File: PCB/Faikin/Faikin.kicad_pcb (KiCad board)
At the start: 2 copper layers, 70 x 70 mm, 27 parts, among them J1 1x5, J3 USB-PROG, Q1 BSS138PS, U3 MD8942, U4 ESP32-S3-MINI-1

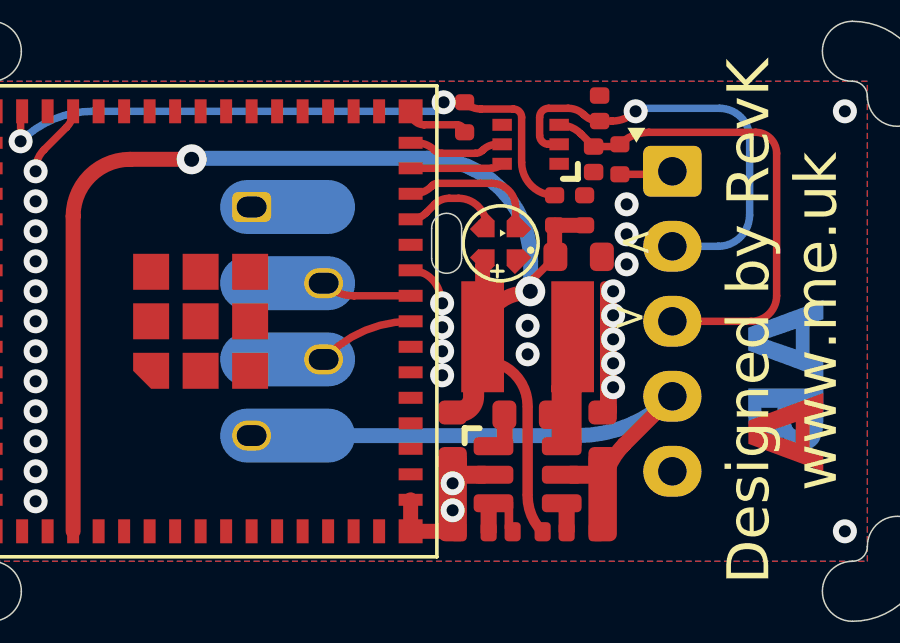
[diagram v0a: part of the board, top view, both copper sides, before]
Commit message: TC2030
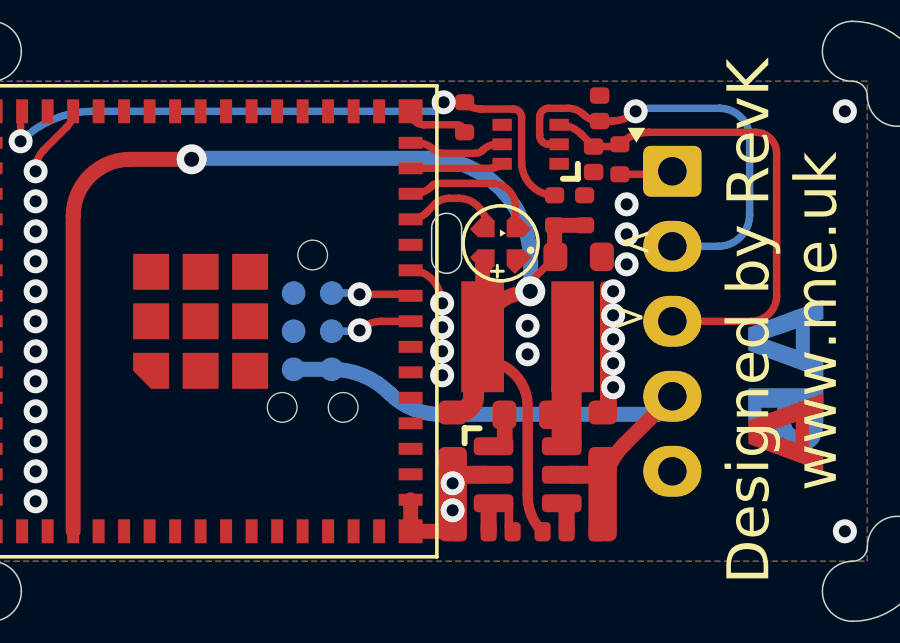
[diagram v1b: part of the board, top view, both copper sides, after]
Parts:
- removed J3: USB-PROG, RevK:USB-PROG2
- added J2: Conn_01x06, RevK:Tag-Connect_TC2030-IDC-NL_2x03_P1.27mm_Vertical, B.Cu at (138.7, 65.3)
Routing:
- net DC: track 16.1 -> 17.5 mm
- net D-: track 3.07 -> 2.72 mm, vias 0 -> 1
- net D+: track 3.01 -> 2.68 mm, vias 0 -> 1
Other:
- board text added: "B"

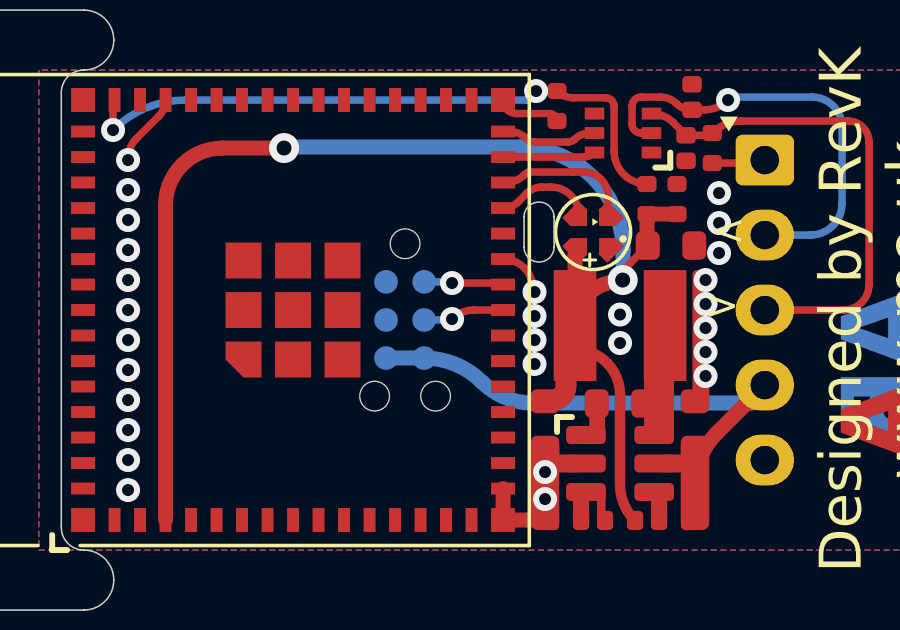
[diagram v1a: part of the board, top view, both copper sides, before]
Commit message: TC2030-USB-NL cable pin out
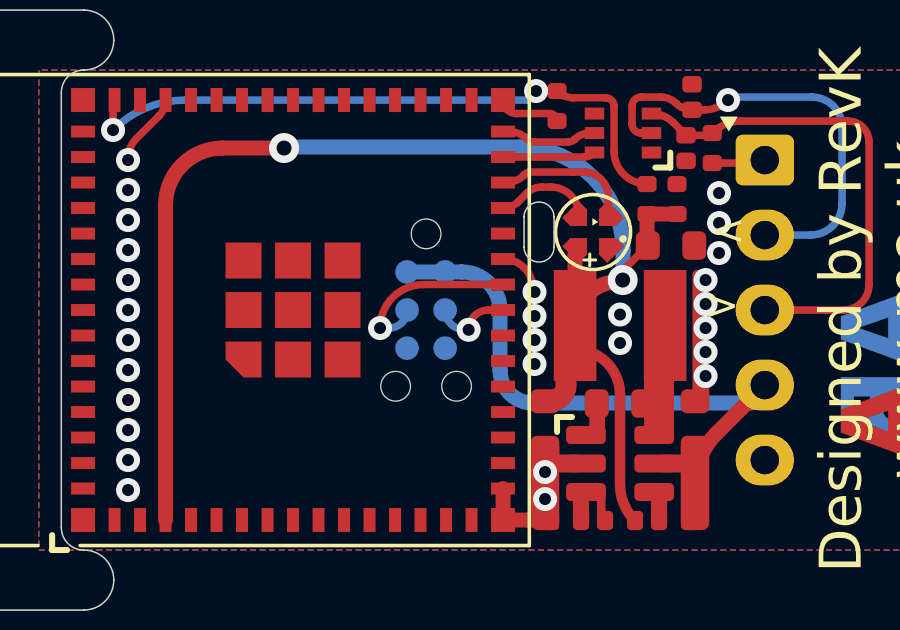
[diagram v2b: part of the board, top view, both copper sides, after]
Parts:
- removed J2: Conn_01x06, RevK:Tag-Connect_TC2030-IDC-NL_2x03_P1.27mm_Vertical
- added J3: TC2030-USB-NL, RevK:Tag-Connect_TC2030-IDC-NL_2x03_P1.27mm_Vertical, B.Cu at (139.4, 65.0)
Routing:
- net D+: track 2.68 -> 6.09 mm
- net DC: track 17.5 -> 19.7 mm
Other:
- board text added: "U"
